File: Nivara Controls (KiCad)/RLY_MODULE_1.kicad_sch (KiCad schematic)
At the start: 0 parts

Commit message: Actualización_RLAY
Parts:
- added U1: LK1802, EastEDA:LK1802, symbol EDA:LK1802
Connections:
- new net +3.3V: U1.5 (COM)
- new net GND: U1.2 (E)
- new net ON_RLY_1: U1.3 (1B)
- new net ON_RLY_2: U1.4 (2B)

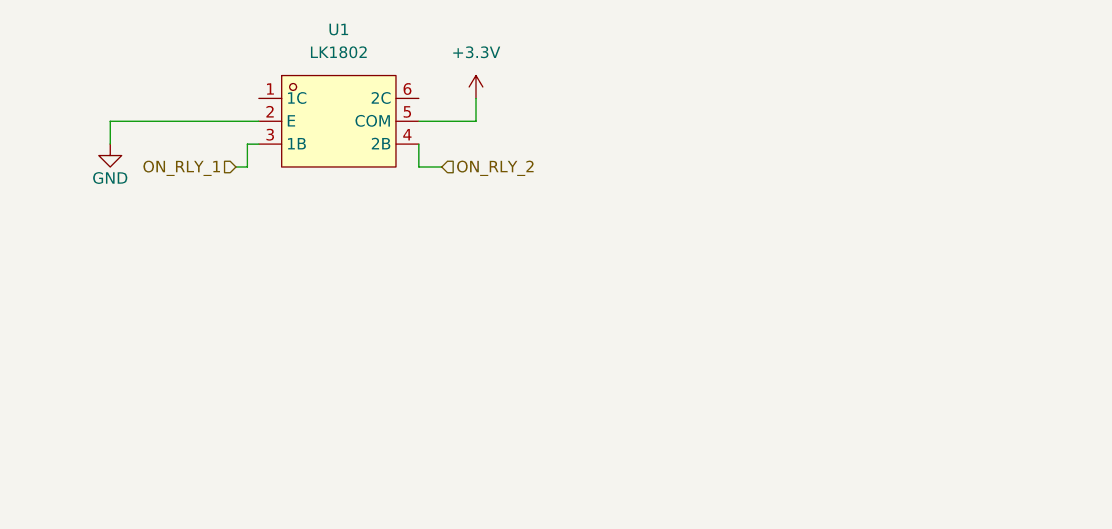
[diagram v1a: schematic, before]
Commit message: Actualization
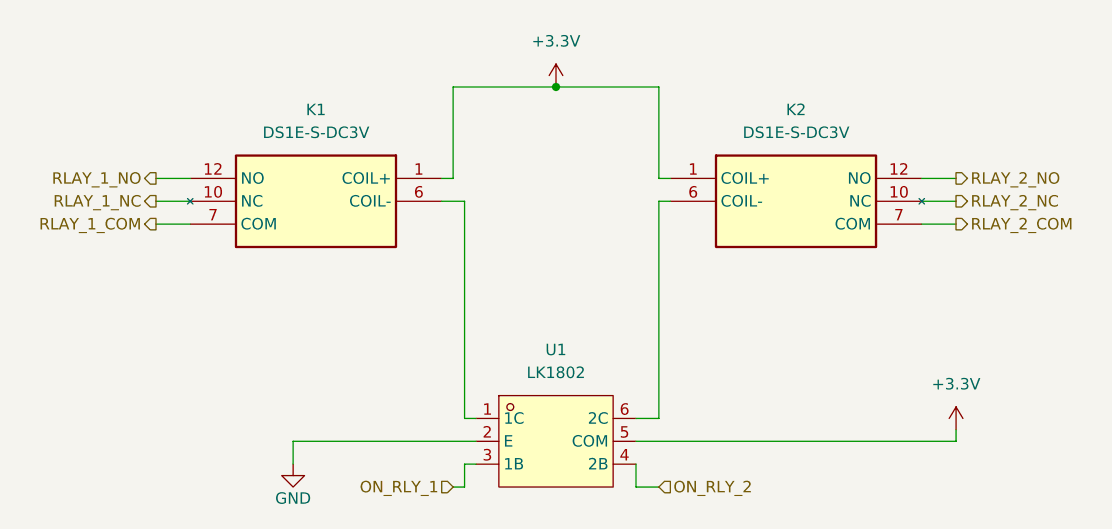
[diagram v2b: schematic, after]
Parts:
- added K1, K2: DS1E-S-DC3V, footprints:RELAY_DS1E_PAN, symbol DS1E-S-DC3V:DS1E-S-DC3V
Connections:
- net +3.3V: now also K1.1 (COIL+), K2.1 (COIL+)
- net at U1.1 (1C): now also K1.6 (COIL-)
- net at U1.6 (2C): now also K2.6 (COIL-)
- new net RLAY_1_COM: K1.7 (COM)
- new net RLAY_1_NC: K1.10 (NC)
- new net RLAY_1_NO: K1.12 (NO)
- new net RLAY_2_COM: K2.7 (COM)
- new net RLAY_2_NC: K2.10 (NC)
- new net RLAY_2_NO: K2.12 (NO)
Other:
- moved on the sheet: U1
